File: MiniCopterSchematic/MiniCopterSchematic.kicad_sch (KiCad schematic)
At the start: 15 parts

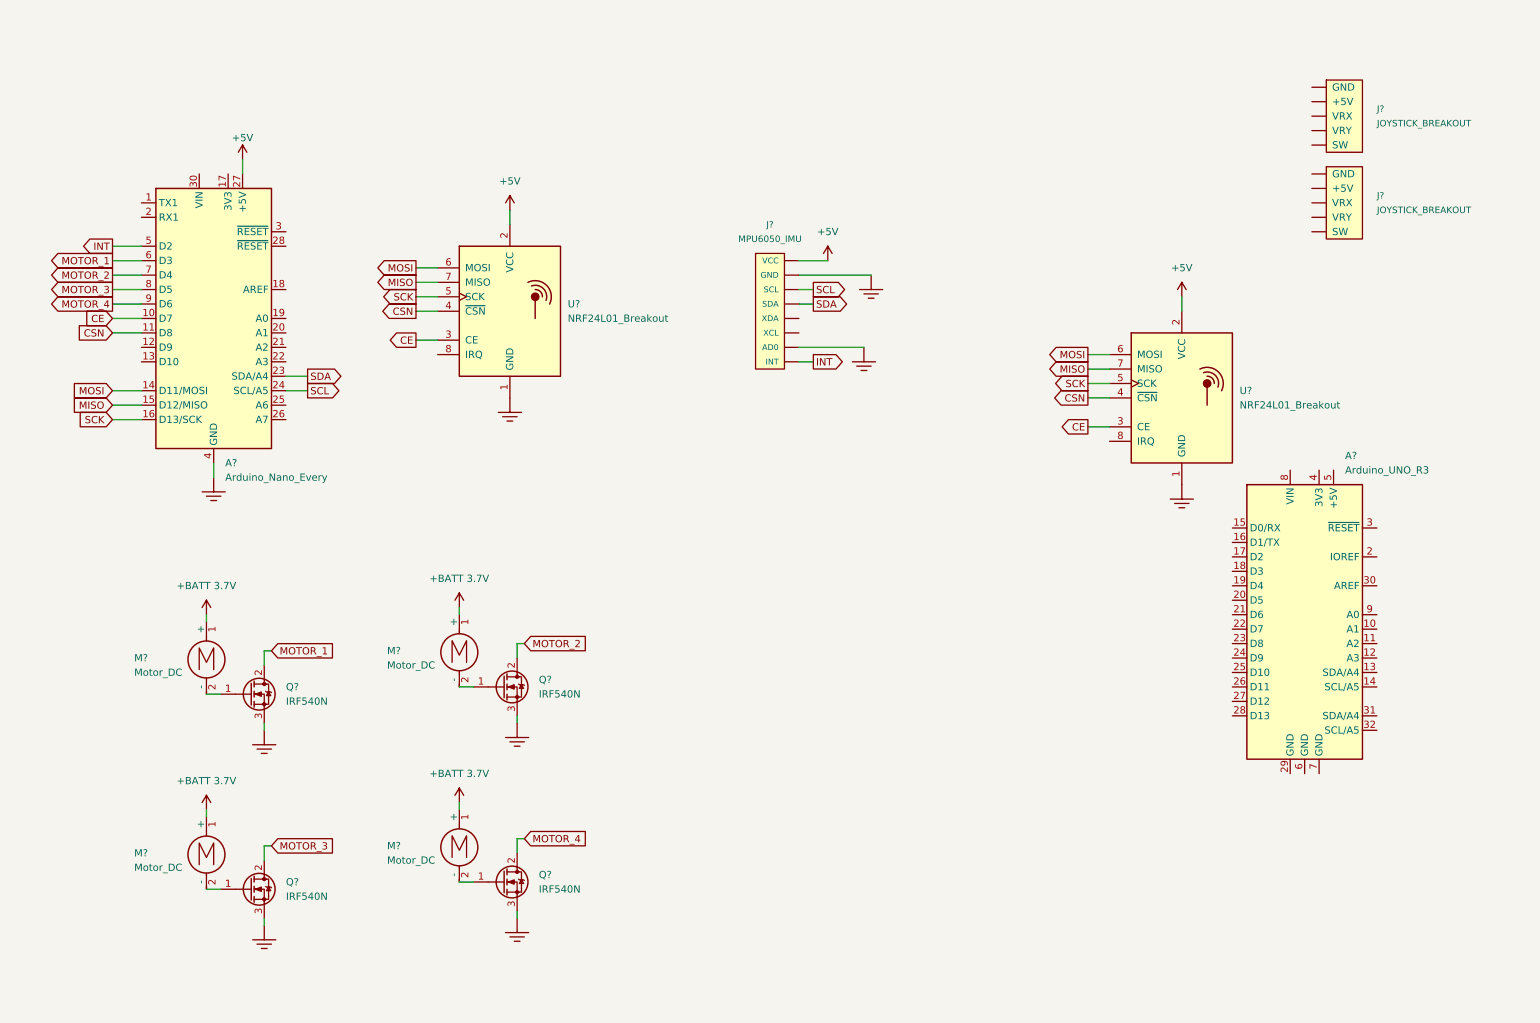
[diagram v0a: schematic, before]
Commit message: Updating schematic
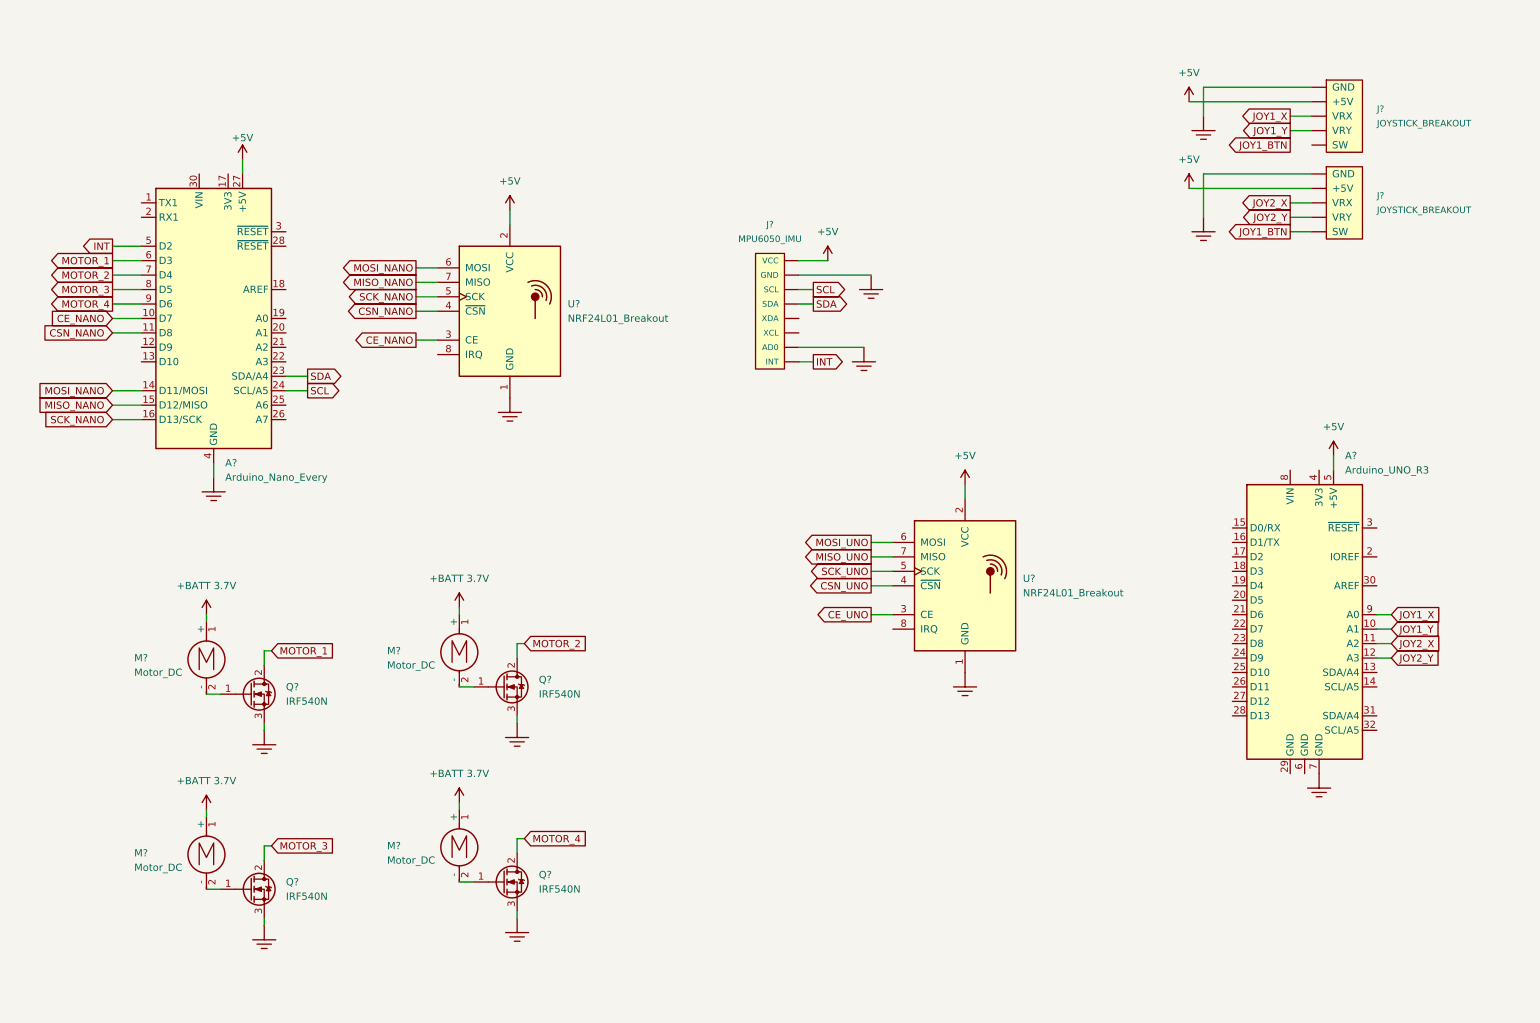
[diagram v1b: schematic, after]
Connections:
- net +BATT: now also A?.5 (+5V), J?.~ (VRY), J?.~ (VRY)
- net GND: now also A?.7 (GND), J?.~ (VRY), J?.~ (VRY)
- net JOY2_Y: now reaches J?.~ (VRY)
- net JOY2_Y: now also A?.12 (A3)
- net JOY1_Y: now reaches A?.10 (A1)
- net JOY1_Y: now also J?.~ (VRY)
- net JOY2_X: now reaches A?.11 (A2)
- net JOY2_X: now also J?.~ (VRY)
- net JOY1_X: now reaches A?.9 (A0)
- net JOY1_X: now also J?.~ (VRY)
- net CE renamed CE_NANO
- net CE_NANO: no longer U?.3 (CE)
- net CSN renamed CSN_NANO
- net CSN_NANO: no longer U?.4 (~{CSN})
- net MISO renamed MISO_NANO
- net MISO_NANO: no longer U?.7 (MISO)
- net MOSI renamed MOSI_NANO
- net MOSI_NANO: no longer U?.6 (MOSI)
- net SCK renamed SCK_NANO
- net SCK_NANO: no longer U?.5 (SCK)
- new net CE_UNO: U?.3 (CE)
- new net CSN_UNO: U?.4 (~{CSN})
- new net JOY1_BTN: J?.~ (VRY)
- new net MISO_UNO: U?.7 (MISO)
- new net MOSI_UNO: U?.6 (MOSI)
- new net SCK_UNO: U?.5 (SCK)
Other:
- moved on the sheet: U?

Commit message: Finished Schematic
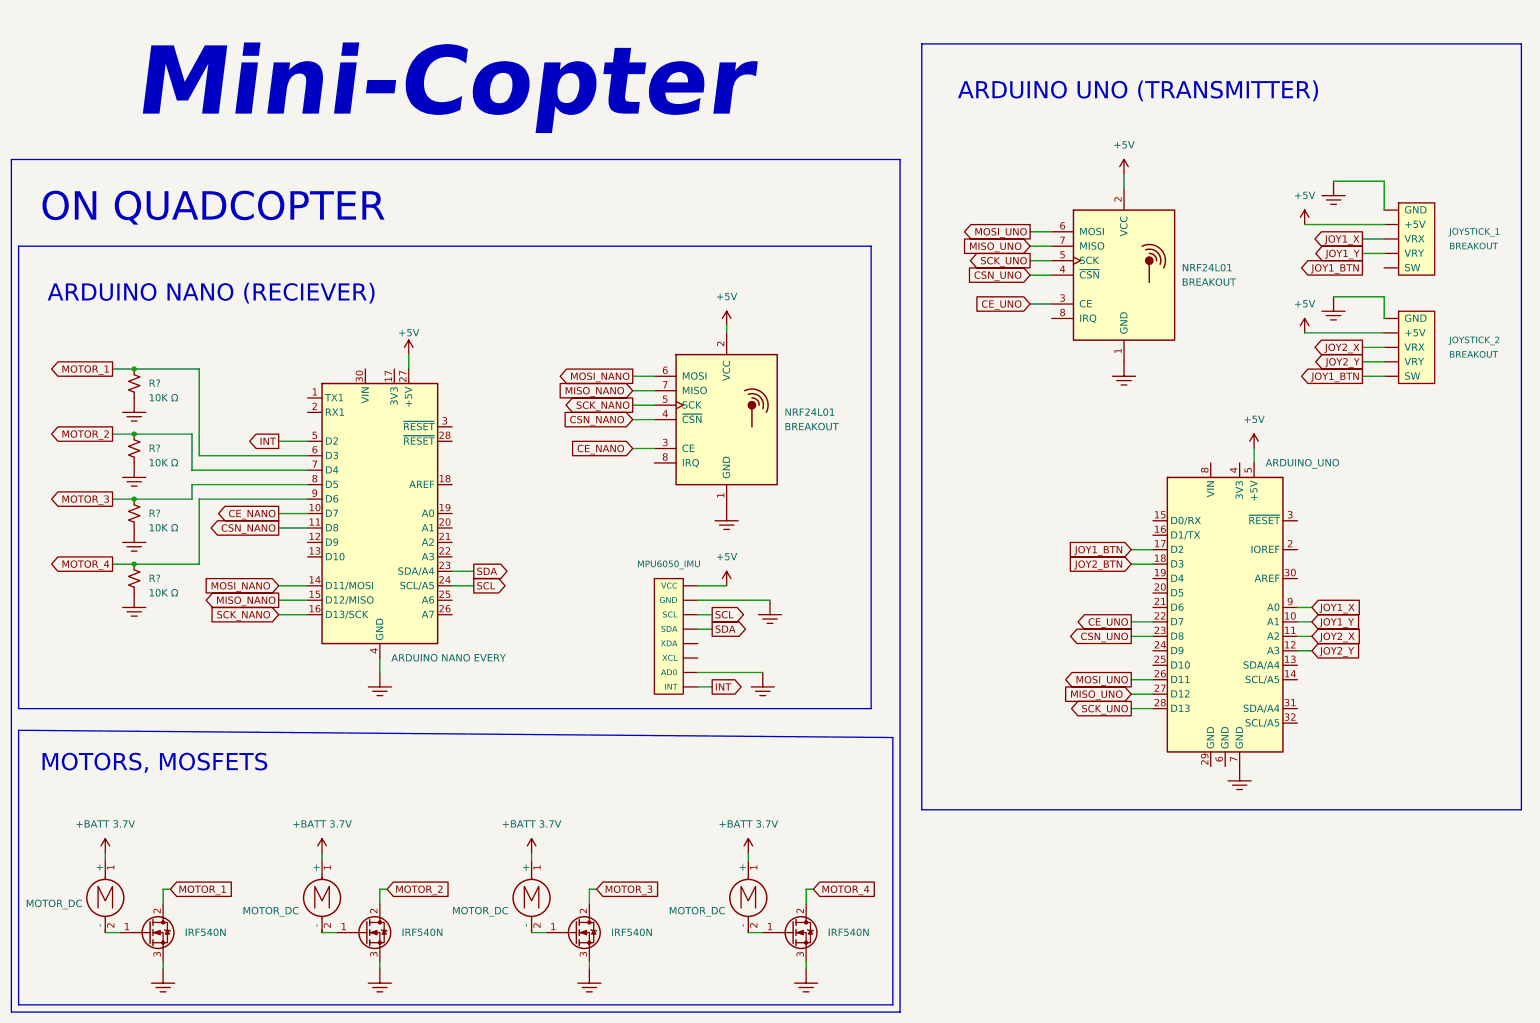
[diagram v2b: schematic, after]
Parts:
- added R? (x4): 10K Ω, symbol Device:R_Small_US
- A?: value Arduino_Nano_Every -> ARDUINO NANO EVERY
- JOYSTICK_1, JOYSTICK_2: renamed from J?; value JOYSTICK_BREAKOUT -> BREAKOUT
- M? (x4): value Motor_DC -> MOTOR_DC
- NRF24L01: renamed from U?; value NRF24L01_Breakout -> BREAKOUT
- ss: renamed from A?; value Arduino_UNO_R3 -> ARDUINO_UNO
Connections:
- net CE_UNO: now also ss.22 (D7)
- net CSN_UNO: now also ss.23 (D8)
- net GND: now also R?.2, R?.2, R?.2, R?.2
- net JOY1_BTN: now also ss.17 (D2)
- net MISO_UNO: now also ss.27 (D12)
- net MOSI_UNO: now also ss.26 (D11)
- net MOTOR_1: now also R?.1
- net MOTOR_2: now also R?.1
- net MOTOR_3: now also R?.1
- net MOTOR_4: now also R?.1
- net SCK_UNO: now also ss.28 (D13)
- net JOY2_BTN: now reaches ss.18 (D3)
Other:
- note added: "ARDUINO NANO (RECIEVER)"
- note added: "ARDUINO UNO (TRANSMITTER)"
- note added: "MOTORS, MOSFETS"
- note added: "Mini-Copter"
- note added: "ON QUADCOPTER"
- title: (none) -> Mini-Copter
- moved on the sheet: JOYSTICK_1, JOYSTICK_2, NRF24L01
